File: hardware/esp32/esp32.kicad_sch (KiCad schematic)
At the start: 42 parts, among them U1 AMS1117-3.3, U2 ESP32-S3-MINI-1-N8, U3 ESD7104MUTAG, U4 BDR6133, U5 TLV75801PDRV

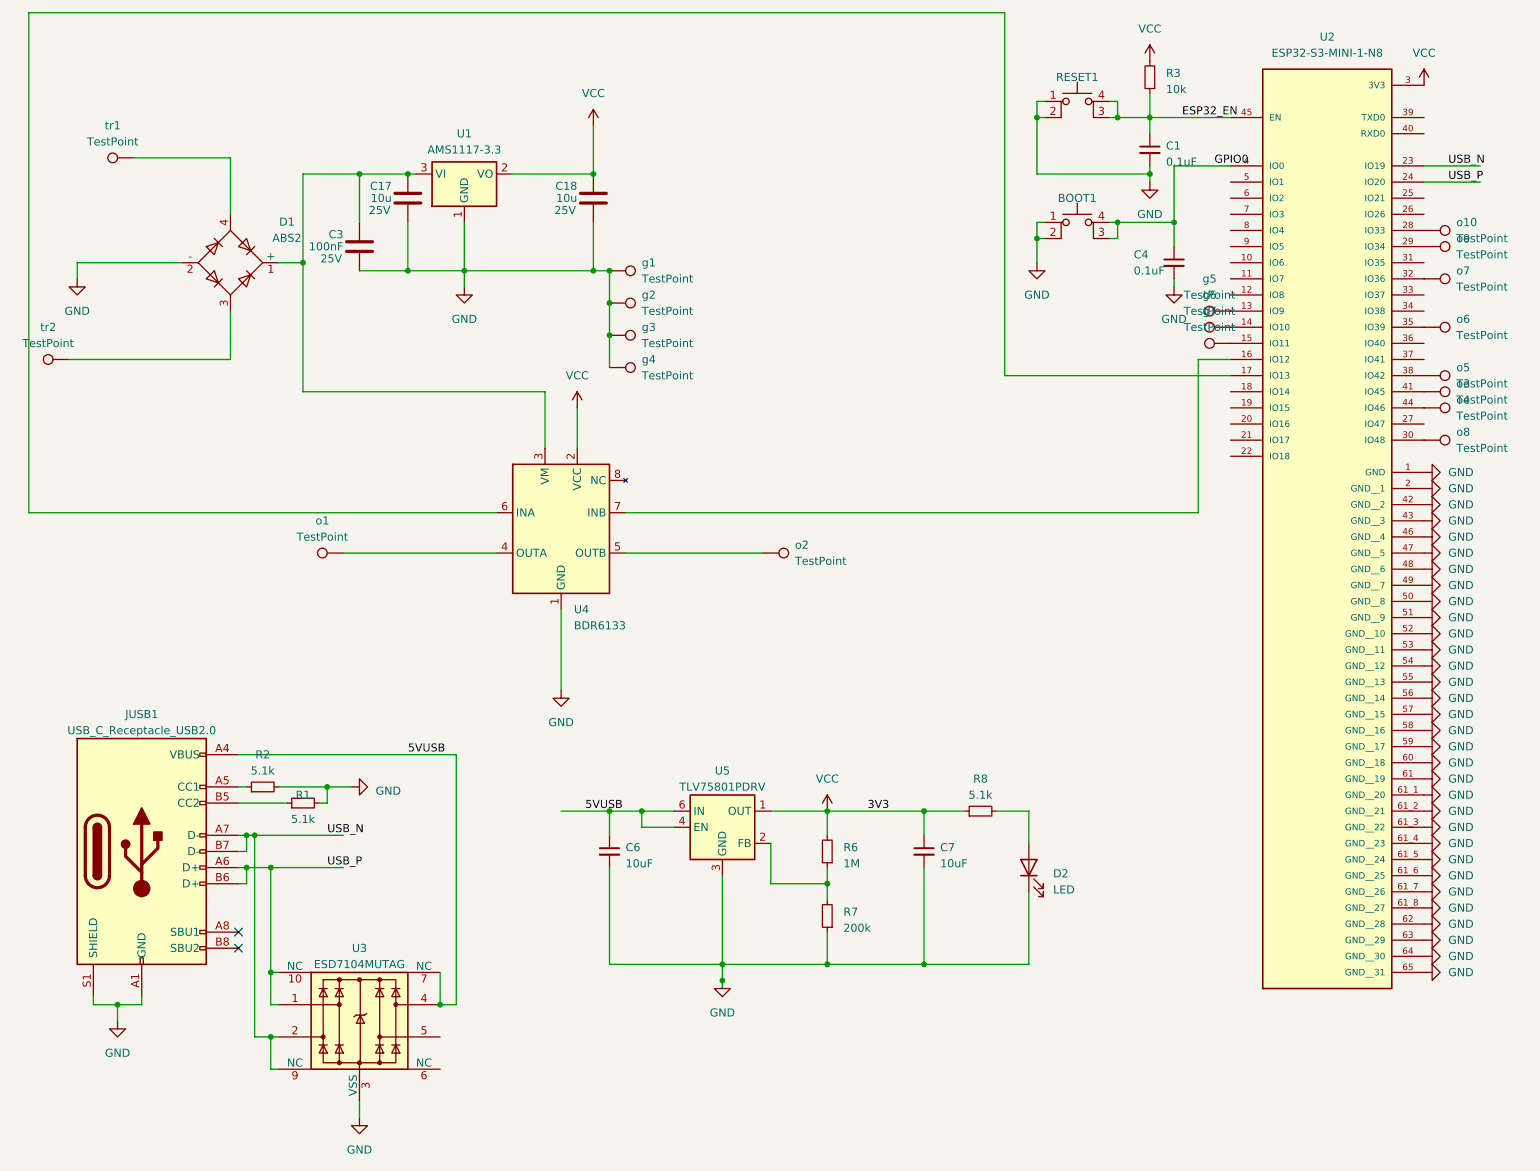
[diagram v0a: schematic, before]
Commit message: TPS629210DRLR
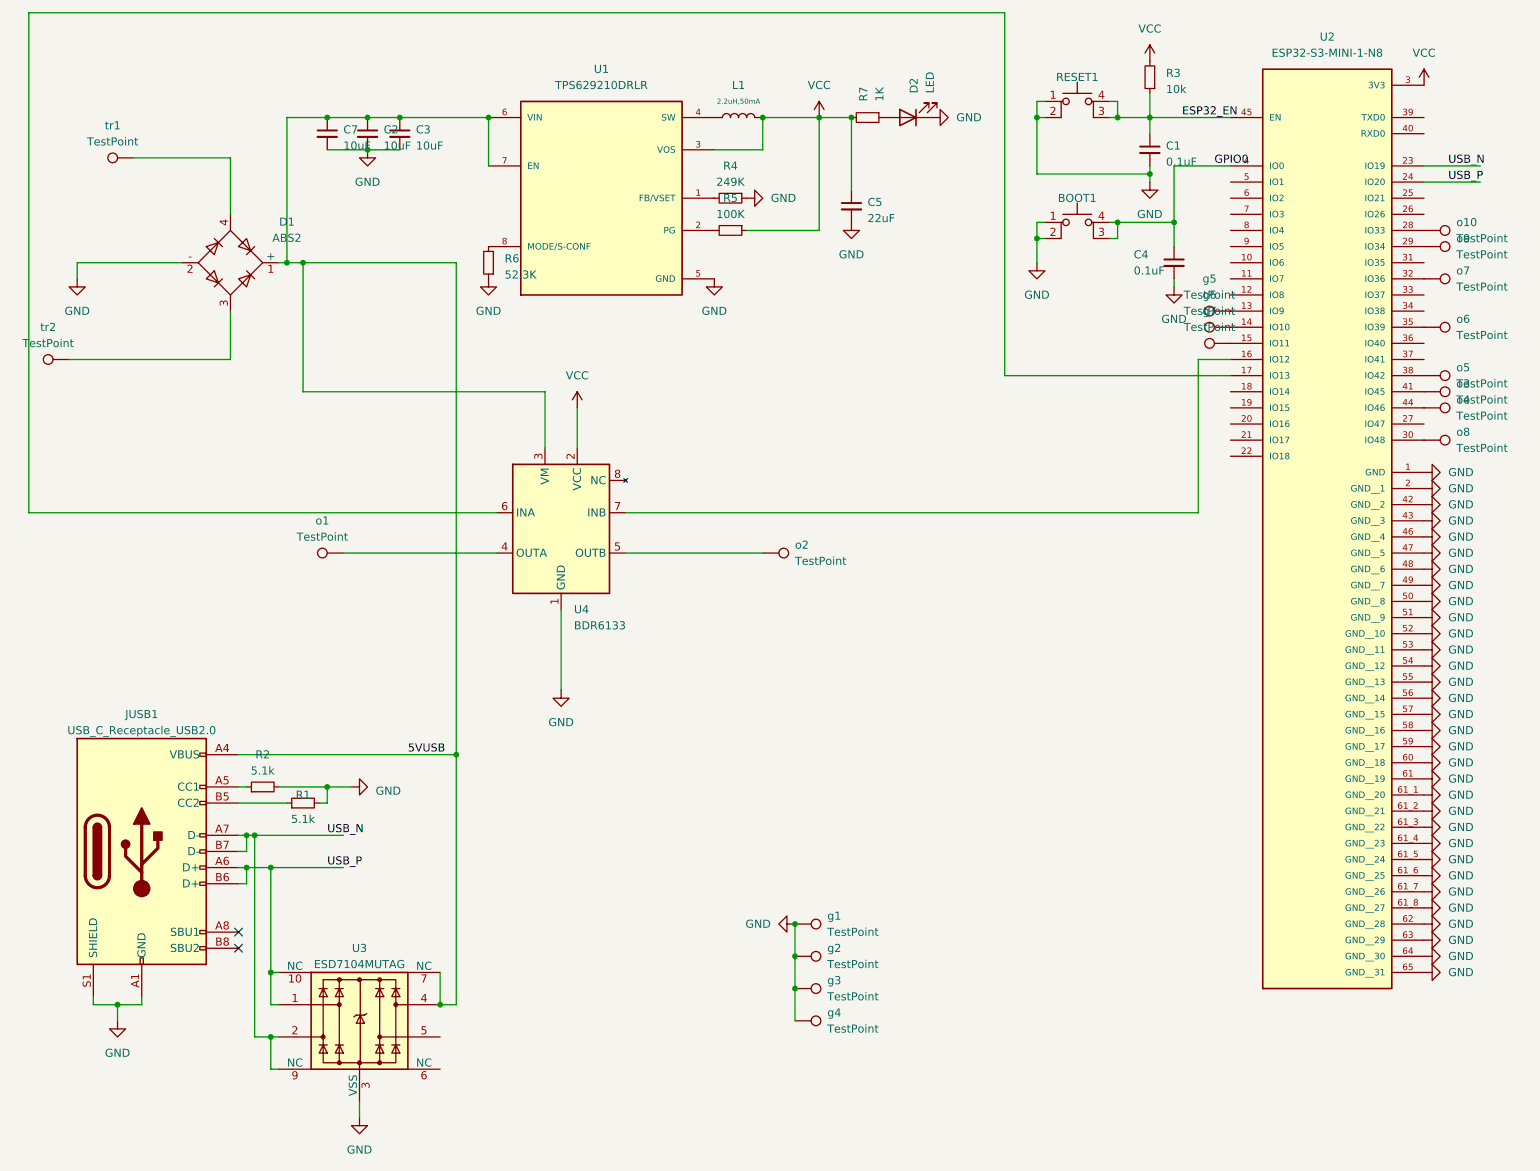
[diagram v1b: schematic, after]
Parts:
- removed C17, C18: 10u, Capacitor_SMD:C_0603_1608Metric, symbol Device:C
- removed C3: 100nF, Capacitor_SMD:C_0603_1608Metric, symbol Device:C
- removed C6: 10uF, Capacitor_SMD:C_0603_1608Metric, symbol Device:C_Small
- removed R8: 5.1k, Resistor_SMD:R_0603_1608Metric, symbol Device:R_Small
- removed U1: AMS1117-3.3, Package_TO_SOT_SMD:SOT-89-3, symbol Regulator_Linear:AMS1117-3.3
- removed U5: TLV75801PDRV, Package_SON:WSON-6-1EP_2x2mm_P0.65mm_EP1x1.6mm, symbol Regulator_Linear:TLV75801PDRV
- added C2, C3: 10uF, Capacitor_SMD:C_0603_1608Metric, symbol Device:C_Small
- added C5: 22uF, Capacitor_SMD:C_0603_1608Metric, symbol Device:C_Small
- added L1: 2.2uH,50mA, PCM_JLCPCB:L_0805, symbol PCM_JLCPCB-Inductors:2.2uH,50mA
- added R4: 249K, Resistor_SMD:R_0603_1608Metric, symbol Device:R_Small
- added R5: 100K, Resistor_SMD:R_0603_1608Metric, symbol Device:R_Small
- added U1: TPS629210DRLR, TPS629210DRLR:SOT50P160X60-8N, symbol TPS629210DRLR:TPS629210DRLR
- R6: value 1M -> 52.3K
- R7: value 200k -> 1K
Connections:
- net 5VUSB: now also C7.1, D1.1 (+), U4.3 (VM), C2.1, C3.1, U1.6 (VIN), U1.7 (EN)
- net GND: now also R6.1, C2.2, C3.2, C5.2, R4.1, U1.5 (GND); no longer R7.1
- net VCC: now also R7.2, C5.1, L1.2, R5.1, U1.3 (VOS); no longer C7.1, R6.2
- net at D2.2 (A): now also R7.1
- new net: R4.2, U1.1 (FB/VSET)
- new net: R5.2, U1.2 (PG)
- new net: R6.2, U1.8 (MODE/S-CONF)
- new net: L1.1, U1.4 (SW)
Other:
- moved on the sheet: C7, D2, R6, g1, g2, g3, g4
